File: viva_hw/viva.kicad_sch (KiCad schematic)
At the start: 16 parts, among them M1 Motor_DC, M2 Motor_DC, M3 Motor_DC, M4 Motor_DC, Q1 2N3904, Q2 2N3904, Q3 2N3904, Q4 2N3904, U1 XIAO ESP32C3

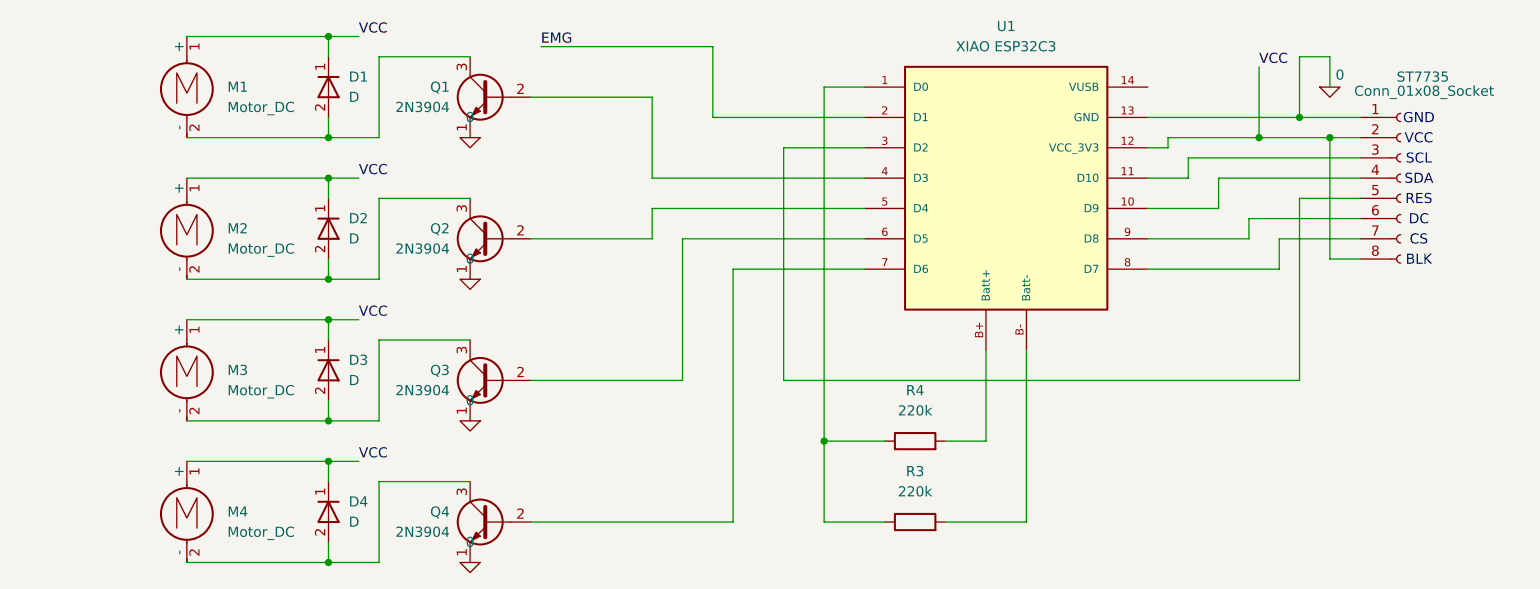
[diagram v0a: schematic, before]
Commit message: feat: updated footprints
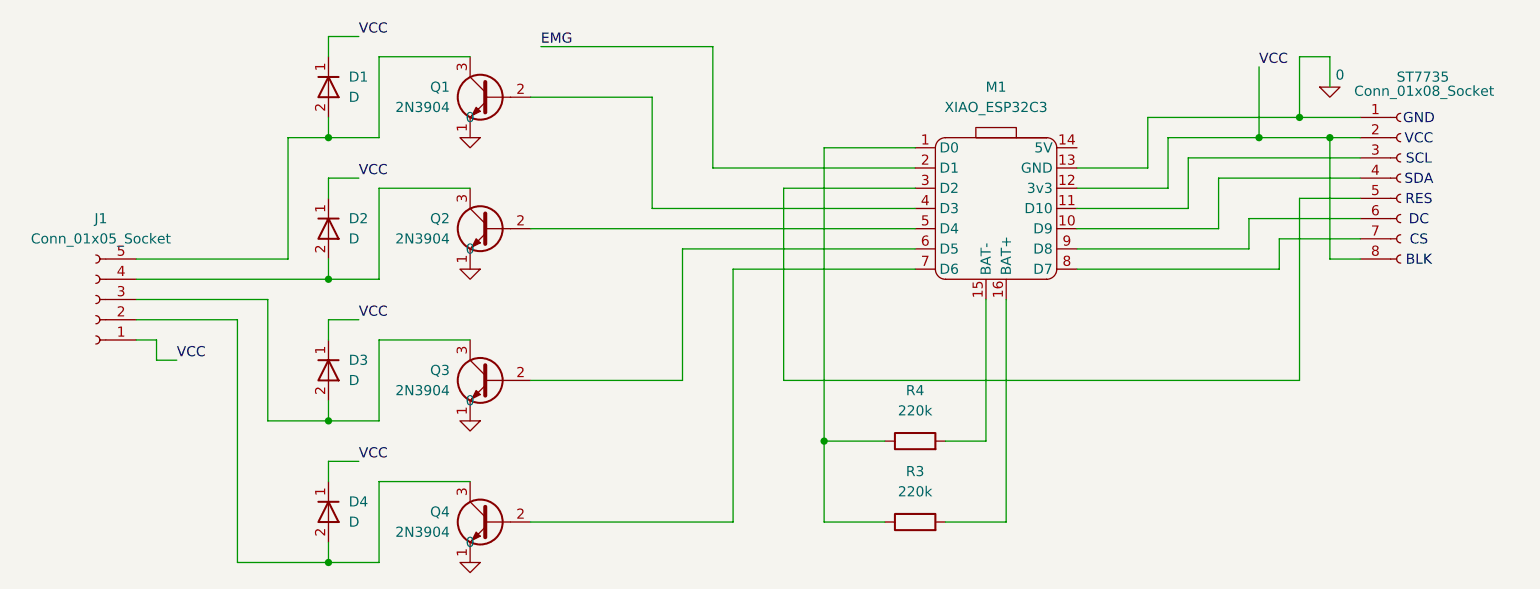
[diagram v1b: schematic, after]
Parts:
- removed M1, M2, M3, M4: Motor_DC, symbol Motor:Motor_DC
- removed U1: XIAO ESP32C3, RF_Module:MCU_Seeed_ESP32C3, symbol xiao_esp32c3:XIAO ESP32C3
- added J1: Conn_01x05_Socket, Connector_PinHeader_2.54mm:PinHeader_1x05_P2.54mm_Vertical, symbol Connector:Conn_01x05_Socket
- added M1: XIAO_ESP32C3, System_On_Chip:XIAO_ESP32C3_THR, symbol System_On_Chip:XIAO_ESP32C3
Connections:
- net 0: now also M1.13 (GND)
- net EMG: now also M1.2 (D1)
- net VCC: now also J1.1 (Pin_1), M1.12 (3v3)
- net at D3.2 (A), Q3.3 (C): now also J1.3 (Pin_3)
- net at D4.2 (A), Q4.3 (C): now also J1.2 (Pin_2)
- net at D2.2 (A), Q2.3 (C): now also J1.4 (Pin_4)
- net at Q3.2 (B): now also M1.6 (D5)
- net at Q2.2 (B): now also M1.5 (D4)
- net at R3.1, R4.1: now also M1.1 (D0)
- net at R3.2: now also M1.16 (BAT+)
- net at R4.2: now also M1.15 (BAT-)
- net at ST7735.4 (Pin_4): now also M1.10 (D9)
- net at ST7735.3 (Pin_3): now also M1.11 (D10)
- net at ST7735.5 (Pin_5): now also M1.3 (D2)
- net at Q1.2 (B): now also M1.4 (D3)
- net at Q4.2 (B): now also M1.7 (D6)
- net at ST7735.7 (Pin_7): now also M1.8 (D7)
- net at ST7735.6 (Pin_6): now also M1.9 (D8)
- net at D1.2 (A), Q1.3 (C): now also J1.5 (Pin_5)
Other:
- moved on the sheet: Q2
